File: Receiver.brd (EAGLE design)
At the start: 53.3 x 63.5 mm, 26 parts, among them IC1 25LC080P, IC2 25LC080P, U1 915MHz, U2 DS3234, X1 BU-SMA-V, X2 53047-05

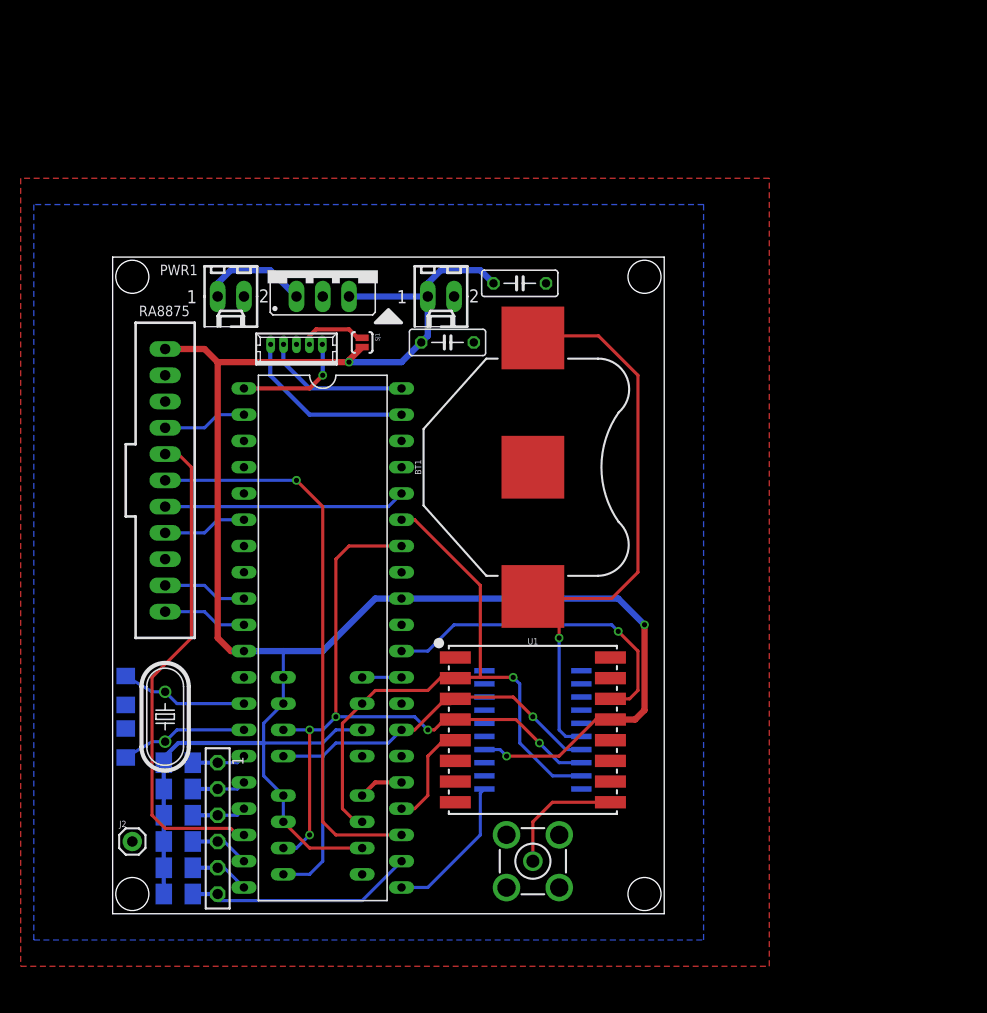
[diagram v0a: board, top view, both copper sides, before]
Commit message: Receiver board r2
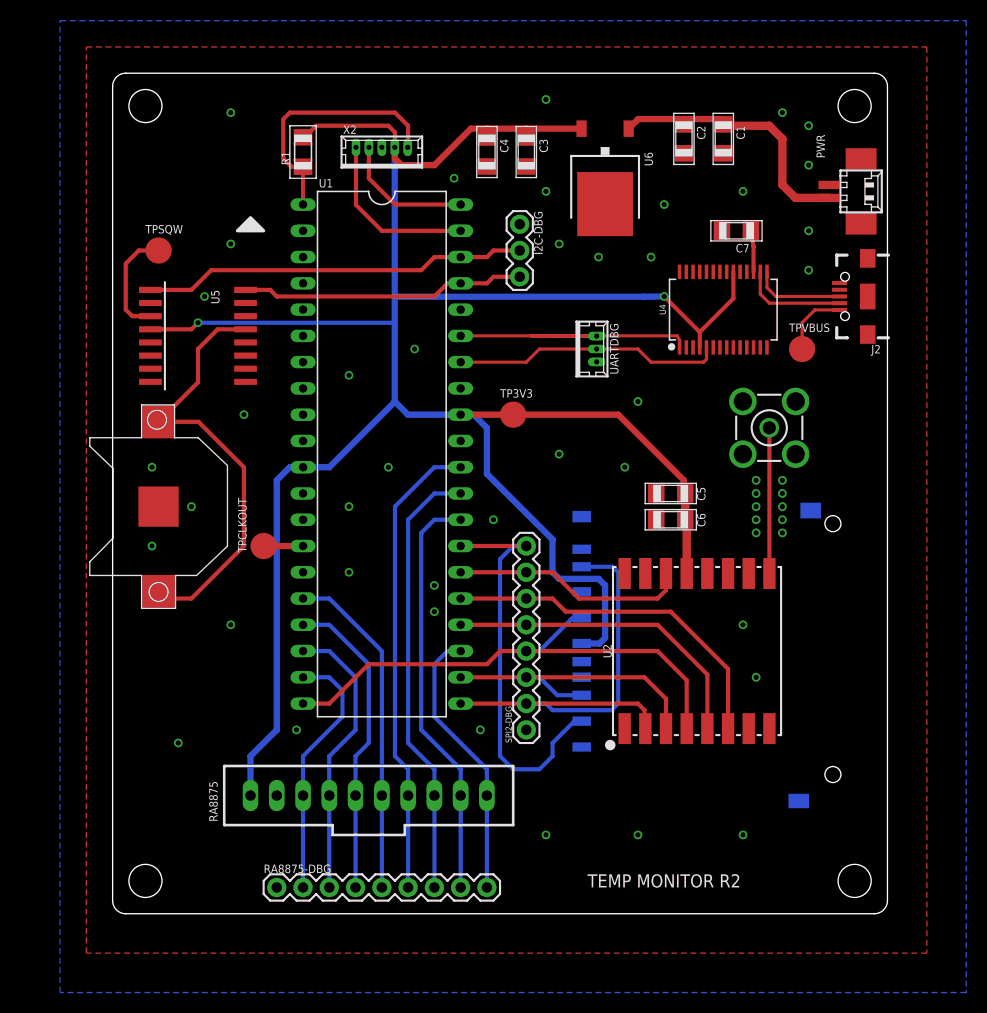
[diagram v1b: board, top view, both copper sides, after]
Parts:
- removed BT1: (no value), SparkFun-Batteries:BATTCON_20MM
- removed BUTTON: TSW-106-02-S-S, con-samtec:TSW-106-02-S-S
- removed IC1, IC2: 25LC080P, microchip:DIL8
- removed IC3: (no value), v-reg:78XXS
- removed PWR1: 22-27-2021-02, con-molex:6410-02
- removed Q1: (no value), crystal:HC49U-V
- removed R2, R3, R4, R5, R6: (no value), resistor:M1206
- removed SJ1: SOLDERJUMPERNO, SparkFun-Retired:SJ_2S-NO
- removed U$1: PIC18F47K40, microchip:DIL40
- added C5, C6: (no value), resistor:C1206
- added C7: 0.1uF, resistor:C1206
- added I2C-DBG: (no value), SparkFun-Connectors:1X03
- added J1: SD_CARD_SOCKET, SparkFun-Connectors:SD
- added RA8875-DBG: (no value), SparkFun-Connectors:1X09
- added SPI2-DBG: (no value), SparkFun-Connectors:1X08
- added TP3V3, TPCLKOUT, TPSQW, TPVBUS: TPB2,54, testpad:B2,54
- added U$3: (no value), adafruit:CR1220-SMD
- added U4: FT232RL, SparkFun-IC-Comms:SSOP28DB
- added U5: DS1374C, FRC696:SO-16DW
- added U6: +12v, SparkFun-IC-Power:TO-252
- added UARTDBG: 53047-03, con-molex:53047-03
- C1: value (none) -> 0.1uF
- C2: value (none) -> 1uF
- C3: value (none) -> 0.1uF; device resistor:C050-025X075 -> resistor:C1206
- C4: value (none) -> 1uF; device resistor:C050-025X075 -> resistor:C1206
- J2: device SparkFun-Connectors:1X01 -> SparkFun-Connectors:USB-B-MICRO-SMD
- PWR: value 22-27-2021-02 -> 53261-02; device con-molex:6410-02 -> con-molex:53261-02
- R1: value (none) -> 10k; device resistor:M1206 -> resistor:R1206
- RA8875: value C-GRID-11-70543 -> C-GRID-10-70543; device con-molex:70543-11 -> con-molex:70543-10
- U1: value 915MHz -> PIC18F47Q84; device SparkFun-RF:RFM69HCW-XXXS2 -> FRC696:DIL40
- U2: value DS3234 -> 915MHz; device SparkFun-Clocks:SO20-0.3 -> SparkFun-RF:RFM69HCW-XXXS2
- X2: value 53047-05 -> PIC-PROG047; device con-molex:53047-05 -> FRC696:53047-05
- moved J2 88.5 mm to (73.0, 59.7), turned to 180 degrees
- moved C1 82.2 mm to (59.1, 74.9), flipped to the top
- moved C2 75.9 mm to (55.2, 74.9), flipped to the top, turned to 270 degrees
- moved R1 60.3 mm to (18.4, 73.7), flipped to the top, turned to 90 degrees
- moved X1 47.7 mm to (63.5, 47.0)
- moved PWR 41.3 mm to (71.8, 69.8), turned to 270 degrees
- moved RA8875 36.3 mm to (24.8, 11.4), turned to 0 degrees
- moved U1 30.4 mm to (26.0, 44.5), turned to 270 degrees
- moved X2 20.8 mm to (26.0, 73.7)
- moved C3 19.9 mm to (40.0, 73.7), turned to 270 degrees
- moved U2 17.6 mm to (56.5, 25.4), flipped to the top
- moved C4 13.1 mm to (36.2, 73.7), turned to 270 degrees
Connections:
- removed net N$14: BT1.1, U2.16
- removed net N$15: U$1.24, U1.5
- removed net N$16: U$1.21, U2.1
- removed net N$17: RA8875.8, U$1.6
- removed net N$18: RA8875.4, U$1.2
- removed net N$19: RA8875.10, U$1.9
- removed net N$20: RA8875.11, U$1.10
- removed net N$21: U$1.30, U1.14
- removed net N$22: SJ1.1, X2.2
- removed net N$23: IC2.1, U$1.25
- removed net N$24: IC3.IN, PWR1.1
- new net CLK_RST: U5.14
- new net RA8875-CS: RA8875-DBG.6, RA8875.7, U1.30
- new net RA8875-INT: RA8875-DBG.9, RA8875.10, U1.23
- new net RA8875-LITE: RA8875-DBG.2, RA8875.3, U1.19
- new net RA8875-RST: RA8875-DBG.7, RA8875.8, U1.29
- new net RA8875-WAIT: RA8875-DBG.8, RA8875.9, U1.28
- new net RF-CS: SPI2-DBG.5, U1.24, U2.5
- new net RF-DIO0: SPI2-DBG.7, U1.26, U2.14
- new net RF-RST: SPI2-DBG.6, U1.25, U2.6
- new net SCL: I2C-DBG.2, U1.38, U5.1
- new net SD-CS: J1.1, SPI2-DBG.8, U1.27
- new net SDA: I2C-DBG.3, U1.37, U5.16
- new net UARTRX: U1.35, U4.1, UARTDBG.3
- new net UARTTX: U1.34, U4.5, UARTDBG.2
- net +3V3: now also C5.1, C6.1, J1.4, TP3V3.TP, U1.11, U1.32, U2.13, U4.20, U4.4, U5.4, U6.2, X2.2; no longer IC1.3, IC1.7, IC1.8, IC2.3, IC2.7, IC2.8, IC3.OUT, PWR.1, R2.2, R3.2, R4.2, R5.2, R6.2, SJ1.2, U$1.11, U$1.32, U1.13, U2.4
- net GND: now also C1.2, C2.2, C5.2, C6.2, C7.2, I2C-DBG.1, J1.3, J1.6, J1.SH@1, J1.SH@2, J2.GND, RA8875-DBG.1, SPI2-DBG.1, U$3.-, U1.12, U1.31, U2.1, U4.18, U4.21, U4.25, U4.26, U4.7, U5.15, U6.3, UARTDBG.1; no longer BT1.2, C1.1, C2.1, IC1.4, IC2.4, IC3.GND, J2.1, PWR1.2, U$1.12, U$1.31, U1.1, U1.10, U1.8, U2.11, U2.12, U2.13, U2.14, U2.15, U2.2, U2.7, U2.9
- net MISO1: now also RA8875-DBG.4, RA8875.5, U1.17; no longer RA8875.6, U$1.23
- net MISO2: now also J1.7, SPI2-DBG.2, U1.21, U2.2; no longer IC1.2, IC2.2, U$1.35, U1.2, U2.19
- net MOSI1: now also RA8875-DBG.5, RA8875.6, U1.16; no longer RA8875.7, U$1.36
- net MOSI2: now also J1.2, SPI2-DBG.3, U1.22, U2.3; no longer IC1.5, IC2.5, U$1.27, U1.3, U2.17
- net N$1: now also U1.39, X2.5; no longer U$1.40, X2.4
- net N$10: now also U$3.+$1, U$3.+$2, U5.13; no longer BUTTON.4, R4.1, U$1.19
- net N$11: now also TPSQW.TP, U5.3; no longer BUTTON.6, R6.1, U$1.22
- net N$12: now also TPCLKOUT.TP, U1.14; no longer IC1.1, U$1.29
- net N$13: now also U2.9; no longer U1.9
- net N$2: now also U1.40, X2.4; no longer U$1.39, X2.5
- net N$3: now also R1.1, U1.1; no longer U$1.1
- net N$4: now also C1.1, C2.1, PWR.1, U6.1; no longer C1.2, Q1.2, U$1.14
- net N$5: now also J2.VBUS, TPVBUS.TP; no longer C2.2, Q1.1, U$1.13
- net N$6: now also C7.1, U4.17; no longer BUTTON.1, R1.1, U$1.15
- net N$7: now also J2.D-, U4.16; no longer BUTTON.2, R2.1, U$1.16
- net N$8: now also J2.D+, U4.15; no longer BUTTON.3, R3.1, U$1.17
- net N$9: now also U1.15; no longer BUTTON.5, R5.1, U$1.20
- net SCK1: now also RA8875-DBG.3, RA8875.4, U1.18; no longer RA8875.5, U$1.18
- net SCK2: now also J1.5, SPI2-DBG.4, U1.20, U2.4; no longer IC1.6, IC2.6, U$1.34, U1.4, U2.18, U2.20
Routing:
- net N$14: track 58.2 -> 0.00 mm, vias 1 -> 0
- net RA8875-CS: track 0.00 -> 45.3 mm
- net RA8875-RST: track 0.00 -> 42.7 mm
- net RA8875-WAIT: track 0.00 -> 40.2 mm
- net SD-CS: track 0.00 -> 39.6 mm
- net SCL: track 0.00 -> 37.3 mm
- net N$10: track 5.74 -> 42.3 mm
- net RF-RST: track 0.00 -> 34.5 mm
- net +3V3: track 207.5 -> 240.9 mm, vias 3 -> 2
- net N$21: track 31.8 -> 0.00 mm, vias 1 -> 0
- net RF-CS: track 0.00 -> 31.1 mm
- net UARTRX: track 0.00 -> 28.5 mm
- net SDA: track 0.00 -> 27.6 mm
- net RA8875-INT: track 0.00 -> 26.8 mm
- net UARTTX: track 0.00 -> 26.1 mm
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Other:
- board size 53.3 x 63.5 mm -> 74.9 x 81.3 mm
- board text added: "TEMP MONITOR R2"
